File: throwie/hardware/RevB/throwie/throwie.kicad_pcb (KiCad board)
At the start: 2 copper layers, 33.8 x 18.8 mm, 24 parts, among them J1 CONN, Q1 2SC3356, Q2 SS8050-G, T1 TestPoints, T2 TestPoints, T3 TestPoints, T4 TestPoints, U1 C8051F850-A-GU, U2 MIC5231-3.3YM5-TR, X1 RO3101

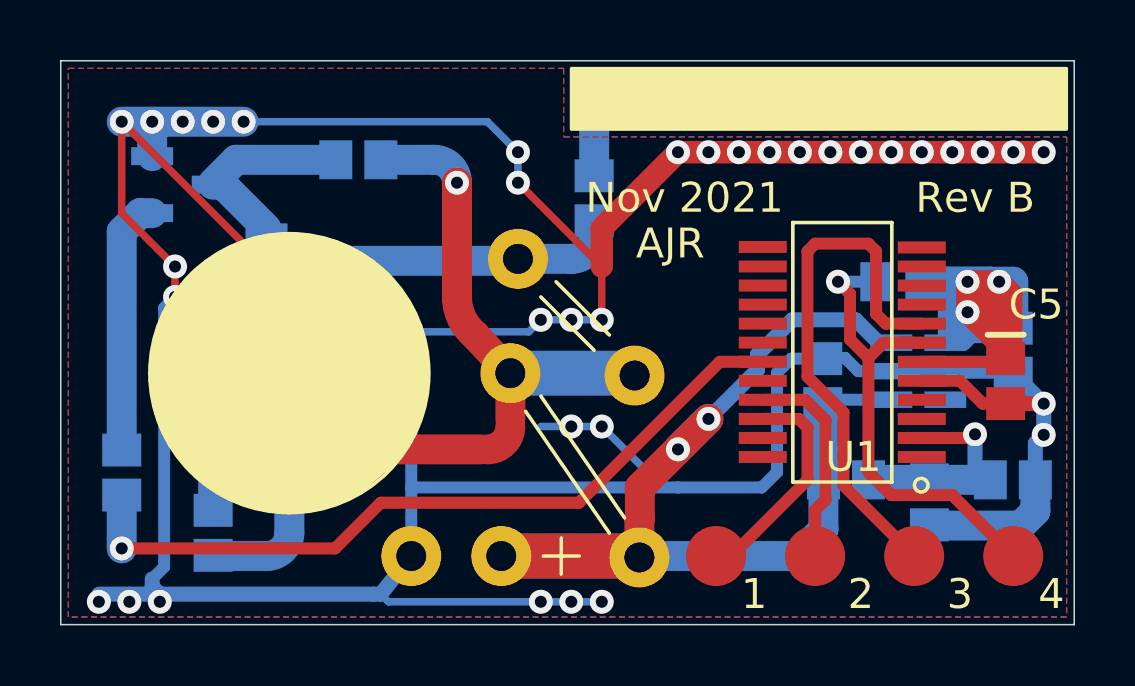
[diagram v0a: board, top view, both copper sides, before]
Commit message: drill file
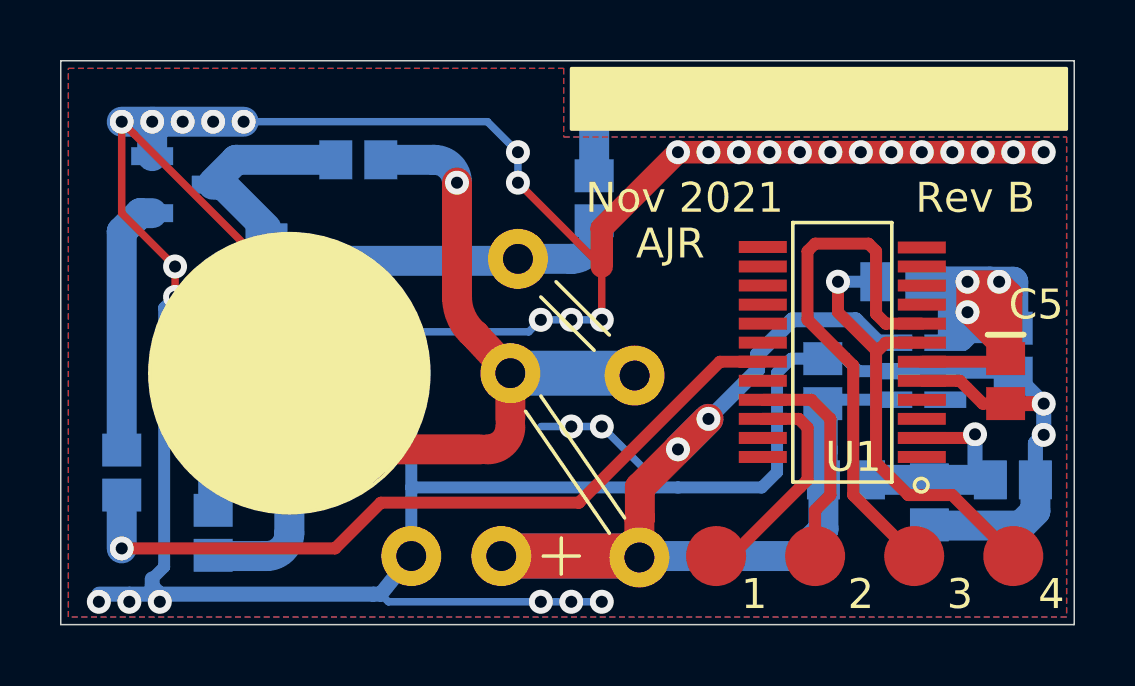
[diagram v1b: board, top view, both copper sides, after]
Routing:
- net Net-(R5-Pad2): track 16.4 -> 15.6 mm
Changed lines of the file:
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@@
     (thickness 1.6)
     (drawings 34)
-    (tracks 270)
+    (tracks 268)
     (zones 0)
     (modules 24)
@@
   (layers
     (0 F.Cu signal)
-    (31 B.Cu signal)
+    (31 B.Cu signal hide)
     (32 B.Adhes user hide)
     (33 F.Adhes user hide)
-    (34 B.Paste user)
+    (34 B.Paste user hide)
     (35 F.Paste user hide)
     (36 B.SilkS user hide)
-    (37 F.SilkS user)
+    (37 F.SilkS user hide)
     (38 B.Mask user hide)
     (39 F.Mask user hide)
@@
   )
   (setup
-    (last_trace_width 1.5)
+    (last_trace_width 0.4)
     (user_trace_width 0.4)
     (user_trace_width 0.5)
@@
   (segment (start 42.545 154.559) (end 37.846 159.258) (width 0.4) (layer F.Cu) (net 11))
   (segment (start 43.976 154.559) (end 42.545 154.559) (width 0.4) (layer F.Cu) (net 11))
-  (segment (start 47.498 158.242) (end 47.498 154.432) (width 0.4) (layer F.Cu) (net 12))
-  (segment (start 47.498 154.432) (end 48.006 153.924) (width 0.4) (layer F.Cu) (net 12))
-  (segment (start 48.006 153.924) (end 49.276 153.924) (width 0.4) (layer F.Cu) (net 12))
   (segment (start 47.498 151.638) (end 47.752 151.892) (width 0.4) (layer B.Cu) (net 12))
-  (segment (start 47.498 158.242) (end 48.26 159.004) (width 0.4) (layer F.Cu) (net 12))
-  (segment (start 50.292 159.004) (end 52.07 160.782) (width 0.4) (layer F.Cu) (net 12))
-  (segment (start 48.26 159.004) (end 50.292 159.004) (width 0.4) (layer F.Cu) (net 12))
-  (segment (start 52.07 160.782) (end 52.324 161.036) (width 0.4) (layer F.Cu) (net 12))
   (via (at 46.482 151.892) (size 0.8) (drill 0.4) (layers F.Cu B.Cu) (net 12))
   (segment (start 47.776 151.892) (end 46.482 151.892) (width 0.4) (layer B.Cu) (net 12))
-  (segment (start 46.881999 153.815999) (end 47.498 154.432) (width 0.4) (layer F.Cu) (net 12))
-  (segment (start 46.881999 152.291999) (end 46.881999 153.815999) (width 0.4) (layer F.Cu) (net 12))
-  (segment (start 46.482 151.892) (end 46.881999 152.291999) (width 0.4) (layer F.Cu) (net 12))
+  (segment (start 48.076 153.924) (end 47.822 154.178) (width 0.4) (layer F.Cu) (net 12))
+  (segment (start 49.276 153.924) (end 48.076 153.924) (width 0.4) (layer F.Cu) (net 12))
+  (segment (start 47.752 157.930002) (end 48.825998 159.004) (width 0.4) (layer F.Cu) (net 12))
+  (segment (start 48.825998 159.004) (end 50.292 159.004) (width 0.4) (layer F.Cu) (net 12))
+  (segment (start 47.752 154.178) (end 47.752 157.930002) (width 0.4) (layer F.Cu) (net 12))
+  (segment (start 50.292 159.004) (end 52.324 161.036) (width 0.4) (layer F.Cu) (net 12))
+  (segment (start 46.482 152.908) (end 47.752 154.178) (width 0.4) (layer F.Cu) (net 12))
+  (segment (start 46.482 151.892) (end 46.482 152.908) (width 0.4) (layer F.Cu) (net 12))
   (segment (start 45.176 156.464) (end 45.466 156.754) (width 0.4) (layer F.Cu) (net 13))
   (segment (start 45.466 158.496) (end 45.212 158.75) (width 0.4) (layer F.Cu) (net 13))
@@
   (segment (start 43.18 160.782) (end 42.926 161.036) (width 0.4) (layer F.Cu) (net 13))
   (segment (start 42.926 161.036) (end 42.418 161.036) (width 0.4) (layer F.Cu) (net 13))
-  (segment (start 46.06601 156.505468) (end 46.06601 159.16599) (width 0.4) (layer F.Cu) (net 14))
-  (segment (start 45.389542 155.829) (end 46.06601 156.505468) (width 0.4) (layer F.Cu) (net 14))
-  (segment (start 43.976 155.829) (end 45.389542 155.829) (width 0.4) (layer F.Cu) (net 14))
-  (segment (start 46.06601 159.16599) (end 45.72 159.512) (width 0.4) (layer F.Cu) (net 14))
+  (segment (start 46.228 156.464) (end 46.228 159.004) (width 0.4) (layer F.Cu) (net 14))
+  (segment (start 46.228 159.004) (end 45.72 159.512) (width 0.4) (layer F.Cu) (net 14))
+  (segment (start 45.593 155.829) (end 46.228 156.464) (width 0.4) (layer F.Cu) (net 14))
   (segment (start 45.72 159.512) (end 45.72 161.036) (width 0.4) (layer F.Cu) (net 14))
-  (segment (start 46.666019 156.256935) (end 46.66602 158.68002) (width 0.4) (layer F.Cu) (net 15))
-  (segment (start 45.466 155.056916) (end 46.666019 156.256935) (width 0.4) (layer F.Cu) (net 15))
-  (segment (start 46.66602 158.68002) (end 49.022 161.036) (width 0.4) (layer F.Cu) (net 15))
-  (segment (start 45.466 150.876) (end 45.466 155.056916) (width 0.4) (layer F.Cu) (net 15))
-  (segment (start 45.72 150.622) (end 45.466 150.876) (width 0.4) (layer F.Cu) (net 15))
-  (segment (start 49.276 153.289) (end 48.076 153.289) (width 0.4) (layer F.Cu) (net 15))
-  (segment (start 47.752 150.876) (end 47.498 150.622) (width 0.4) (layer F.Cu) (net 15))
-  (segment (start 47.752 152.965) (end 47.752 150.876) (width 0.4) (layer F.Cu) (net 15))
-  (segment (start 48.076 153.289) (end 47.752 152.965) (width 0.4) (layer F.Cu) (net 15))
-  (segment (start 47.498 150.622) (end 45.72 150.622) (width 0.4) (layer F.Cu) (net 15))
+  (segment (start 43.976 155.829) (end 45.593 155.829) (width 0.4) (layer F.Cu) (net 14))
+  (segment (start 48.076 153.289) (end 49.276 153.289) (width 0.4) (layer F.Cu) (net 15))
+  (segment (start 47.752 152.965) (end 48.076 153.289) (width 0.4) (layer F.Cu) (net 15))
+  (segment (start 47.752 150.876) (end 47.752 152.965) (width 0.4) (layer F.Cu) (net 15))
+  (segment (start 47.498 150.622) (end 47.752 150.876) (width 0.4) (layer F.Cu) (net 15))
+  (segment (start 45.72 150.622) (end 47.498 150.622) (width 0.4) (layer F.Cu) (net 15))
+  (segment (start 46.99 159.004) (end 46.99 154.686) (width 0.4) (layer F.Cu) (net 15))
+  (segment (start 45.466 153.162) (end 45.466 150.876) (width 0.4) (layer F.Cu) (net 15))
+  (segment (start 46.99 154.686) (end 45.466 153.162) (width 0.4) (layer F.Cu) (net 15))
+  (segment (start 45.466 150.876) (end 45.72 150.622) (width 0.4) (layer F.Cu) (net 15))
+  (segment (start 49.022 161.036) (end 46.99 159.004) (width 0.4) (layer F.Cu) (net 15))
   (zone (net 0) (net_name "") (layer B.Cu) (hatch edge 0.508)
     (connect_pads (clearance 0.508))
